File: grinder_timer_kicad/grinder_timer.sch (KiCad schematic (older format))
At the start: 24 parts, among them IC1 ATMEGA328P-P, U1 SSD1306_128x64OLED, U2 serial_to_usb

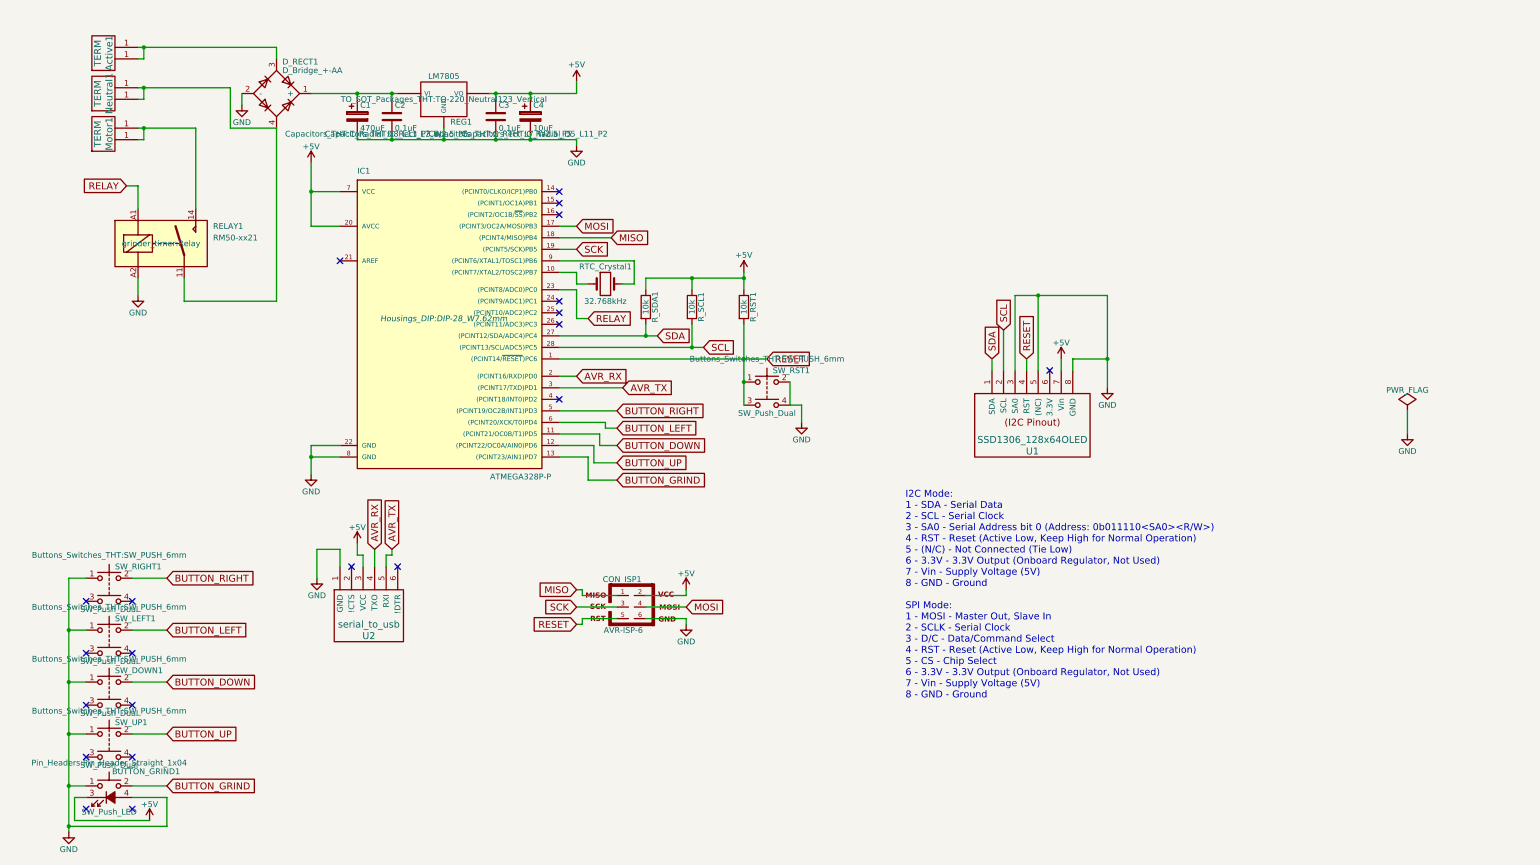
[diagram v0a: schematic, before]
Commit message: Worked on the schematic and footprints.
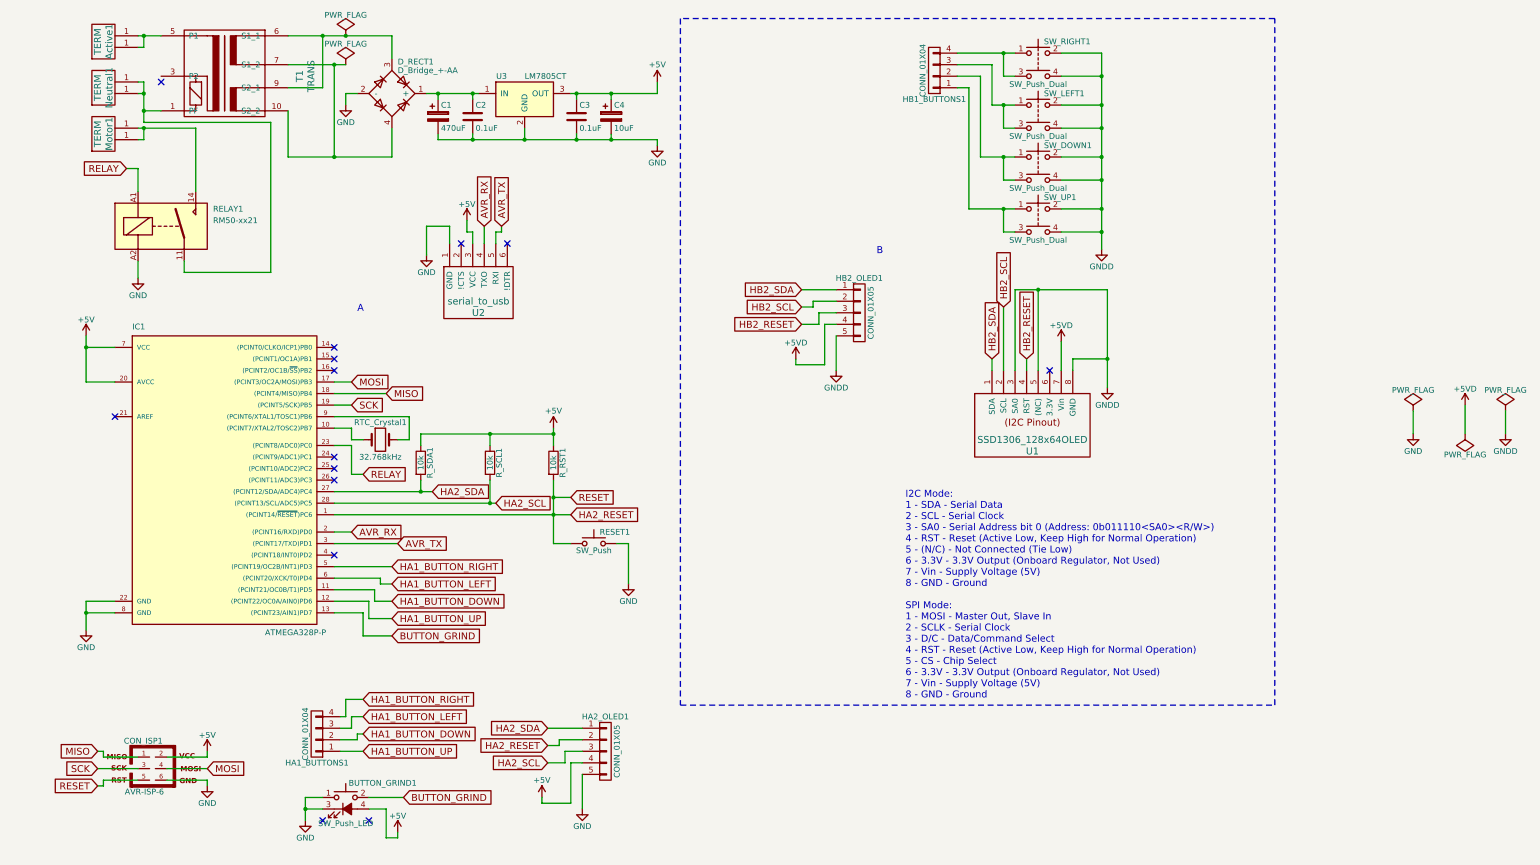
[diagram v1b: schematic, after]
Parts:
- removed REG1: LM7805, TO_SOT_Packages_THT:TO-220_Neutral123_Vertical, symbol LM7805
- removed SW_RST1: SW_Push_Dual, Buttons_Switches_THT:SW_PUSH_6mm, symbol SW_Push_Dual
- added HA1_BUTTONS1, HB1_BUTTONS1: CONN_01X04, Pin_Headers:Pin_Header_Straight_1x04, symbol CONN_01X04
- added HA2_OLED1, HB2_OLED1: CONN_01X05, Pin_Headers:Pin_Header_Straight_1x05, symbol CONN_01X05
- added RESET1: SW_Push, Buttons_Switches_THT:SW_PUSH_6mm, symbol SW_Push
- added T1: TRANS, grinder_timer:TRANS, symbol TRANS
- added U3: LM7805CT, TO-220, symbol LM7805CT
- Active1, Motor1, Neutral1: footprint (none) -> grinder_timer:SPADE_LUG
- D_RECT1: footprint (none) -> grinder_timer:BRIDGE_RECT
- RELAY1: footprint grinder_timer:Relay -> grinder_timer:RELAY
- R_RST1, R_SCL1, R_SDA1: footprint (none) -> Resistors_THT:Resistor_Horizontal_RM10mm
- SW_DOWN1, SW_LEFT1, SW_RIGHT1, SW_UP1: footprint Buttons_Switches_THT:SW_PUSH_6mm -> grinder_timer:TACT
- U1: footprint (none) -> grinder_timer:OLED
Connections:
- net +5V: now also BUTTON_GRIND1.4 (A), HA2_OLED1.4 (P4), U3.3 (OUT); no longer BUTTON_GRIND1.3 (K), U1.7 (Vin)
- net GND: now also BUTTON_GRIND1.3 (K), HA2_OLED1.5 (P5), RESET1.2, U3.2 (GND); no longer BUTTON_GRIND1.4 (A), SW_DOWN1.1, SW_LEFT1.1, SW_RIGHT1.1, SW_UP1.1, U1.3 (SA0), U1.5 ((NC)), U1.8 (GND)
- net at SW_DOWN1.3: now also SW_DOWN1.1, HB1_BUTTONS1.2 (P2)
- net GNDD: now reaches SW_DOWN1.4
- net GNDD: now also SW_DOWN1.2, SW_LEFT1.2, SW_LEFT1.4, SW_RIGHT1.2, SW_RIGHT1.4, SW_UP1.2, SW_UP1.4, U1.3 (SA0), U1.5 ((NC)), U1.8 (GND), HB2_OLED1.5 (P5)
- net at SW_UP1.3: now also SW_UP1.1, HB1_BUTTONS1.1 (P1)
- net at SW_LEFT1.3: now also SW_LEFT1.1, HB1_BUTTONS1.3 (P3)
- net at SW_RIGHT1.3: now also SW_RIGHT1.1, HB1_BUTTONS1.4 (P4)
- net at Neutral1.1, RELAY1.11: now also T1.1 (PF); no longer D_RECT1.4
- net at C1.1, C2.1, D_RECT1.1 (+): now also U3.1 (IN)
- net at D_RECT1.3: now also T1.6 (S1_1), T1.9 (S2_1); no longer Active1.1
- net BUTTON_DOWN renamed HA1_BUTTON_DOWN
- net HA1_BUTTON_DOWN: now also HA1_BUTTONS1.2 (P2); no longer SW_DOWN1.2
- net BUTTON_LEFT renamed HA1_BUTTON_LEFT
- net HA1_BUTTON_LEFT: now also HA1_BUTTONS1.3 (P3); no longer SW_LEFT1.2
- net BUTTON_RIGHT renamed HA1_BUTTON_RIGHT
- net HA1_BUTTON_RIGHT: now also HA1_BUTTONS1.4 (P4); no longer SW_RIGHT1.2
- net BUTTON_UP renamed HA1_BUTTON_UP
- net HA1_BUTTON_UP: now also HA1_BUTTONS1.1 (P1); no longer SW_UP1.2
- net RESET renamed HA2_RESET
- net HA2_RESET: now also HA2_OLED1.2 (P2), RESET1.1; no longer U1.4 (RST)
- net SCL renamed HA2_SCL
- net HA2_SCL: now also HA2_OLED1.3 (P3); no longer U1.2 (SCL)
- net SDA renamed HA2_SDA
- net HA2_SDA: now also HA2_OLED1.1 (P1); no longer U1.1 (SDA)
- new net: D_RECT1.4, T1.10 (S2_2), T1.7 (S1_2)
- new net: Active1.1, T1.5 (P1)
- new net +5VD: HB2_OLED1.4 (P4), U1.7 (Vin)
- new net HB2_RESET: HB2_OLED1.3 (P3), U1.4 (RST)
- new net HB2_SCL: HB2_OLED1.2 (P2), U1.2 (SCL)
- new net HB2_SDA: HB2_OLED1.1 (P1), U1.1 (SDA)
- no-connect marks 21 -> 14
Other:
- note added: "A"
- note added: "B"
- moved on the sheet: Active1, BUTTON_GRIND1, C1, C2, C3, C4, CON_ISP1, D_RECT1, IC1, Neutral1, RELAY1, RTC_Crystal1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
